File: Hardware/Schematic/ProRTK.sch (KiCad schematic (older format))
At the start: 37 parts

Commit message: Add files via upload
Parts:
- removed C? (x2): 1uF, symbol Device:C
- removed U?: AMS1117-3.3, Package_TO_SOT_SMD:SOT-223-3_TabPin2, symbol Regulator_Linear:AMS1117-3.3
- added 1PPS, RX_GNSS?, SCL_ALT, SCL_GNSS, SDA_ALT, SDA_GNSS, SYS_RSTN, TX_GNSS, WAKE-UP: TestPoint, symbol Connector:TestPoint
- added C? (x2): C, symbol Device:C
- added D?: SP0502BAJT, Package_TO_SOT_SMD:SOT-323_SC-70, symbol Power_Protection:SP0502BAJT
- added IC?: ST1S12GR, ASSETS:SOT95P280X110-5N, symbol Regular_Use:ST1S12GR
- added L?: L, symbol Device:L
- added R? (x3): R, symbol Device:R
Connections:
- net labels added: +3V3, 1PPS, RX_GNSS, SCL_ALT, SCL_GNSS, SCL_IMU, SDA_ALT, SDA_GNSS, SDA_IMU, SYS_RSTN, TX_GNSS, WAKE-UP
- net labels removed: SCL, SDA
- wire segments 92 -> 126
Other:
- moved on the sheet: 3.3V, CLK, CMD, CR2023, D+, D-, DAT0, DAT1, DAT2, DAT3, GND, VDD

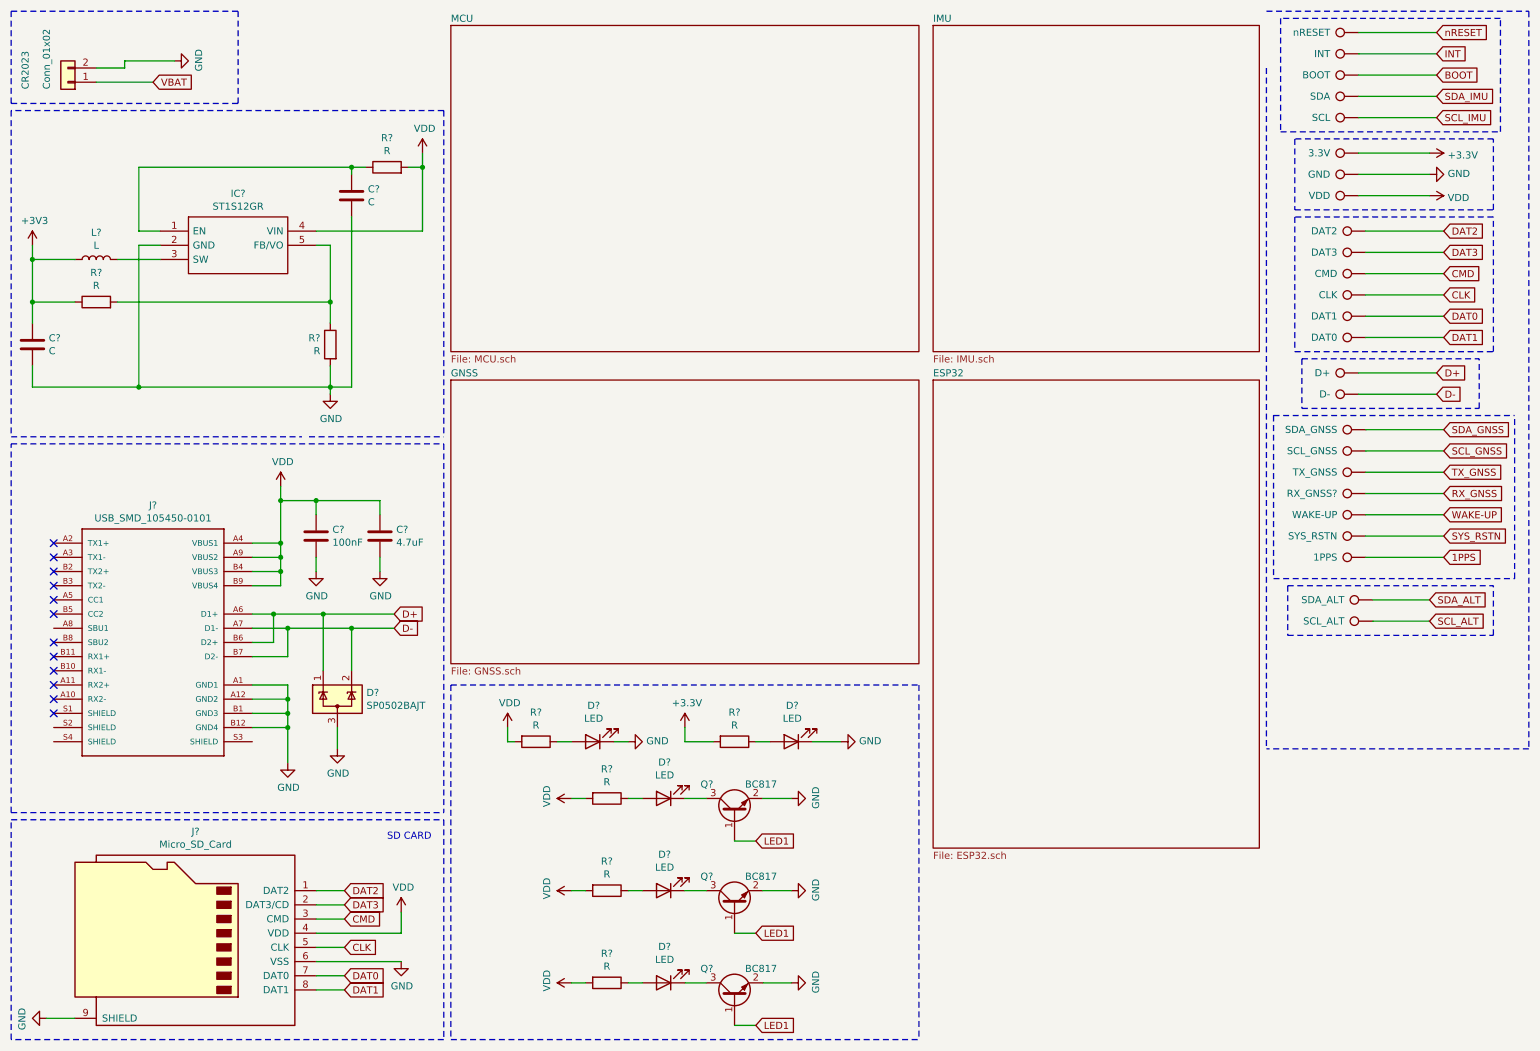
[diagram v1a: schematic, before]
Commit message: Add files via upload
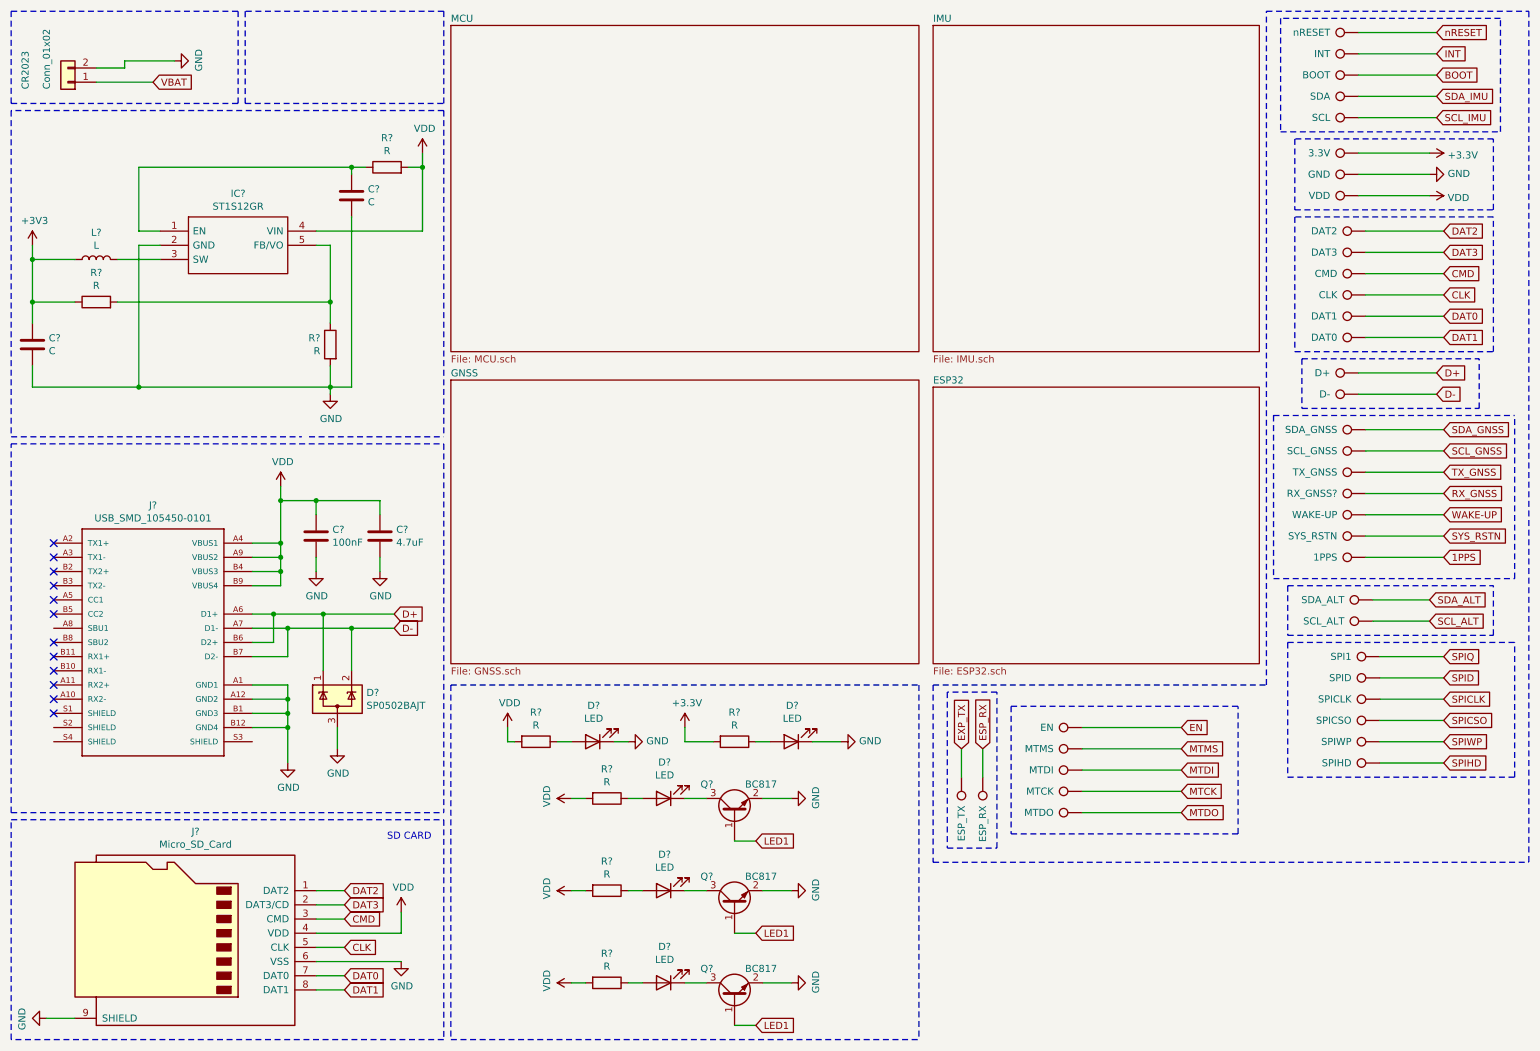
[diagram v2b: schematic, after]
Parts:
- added EN, ESP_RX, ESP_TX, MTCK, MTDI, MTDO, MTMS, SPI1, SPICLK, SPICSO, SPID, SPIHD, SPIWP: TestPoint, symbol Connector:TestPoint
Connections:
- new net EN: EN.1
- new net ESP_RX: ESP_RX.1
- new net EXP_TX: ESP_TX.1
- new net MTCK: MTCK.1
- new net MTDI: MTDI.1
- new net MTDO: MTDO.1
- new net MTMS: MTMS.1
- new net SPICLK: SPICLK.1
- new net SPICSO: SPICSO.1
- new net SPID: SPID.1
- new net SPIHD: SPIHD.1
- new net SPIQ: SPI1.1
- new net SPIWP: SPIWP.1
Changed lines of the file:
@@
 	9500 4550 10950 4550
 Wire Notes Line
-	11200 5700 9350 5700
-Wire Notes Line
-	9350 900  9350 5700
-Wire Notes Line
-	11200 500  11200 5700
+	11200 500  11200 6500
 $Sheet
-S 7000 3100 2300 3300
+S 7000 3150 2300 1950
 U 609C383C
 F0 "ESP32" 50
 F1 "ESP32.sch" 50
 $EndSheet
+Text GLabel 10600 5050 2    50   Input ~ 0
+SPIQ
+Text GLabel 10600 5200 2    50   Input ~ 0
+SPID
+Text GLabel 10600 5350 2    50   Input ~ 0
+SPICLK
+Text GLabel 10600 5500 2    50   Input ~ 0
+SPICSO
+Text GLabel 10600 5800 2    50   Input ~ 0
+SPIHD
+Text GLabel 10600 5650 2    50   Input ~ 0
+SPIWP
+Text GLabel 7200 5700 1    50   Input ~ 0
+EXP_TX
+Text GLabel 7350 5700 1    50   Input ~ 0
+ESP_RX
+Text GLabel 8750 5550 2    50   Input ~ 0
+EN
+Text GLabel 8750 5700 2    50   Input ~ 0
+MTMS
+Text GLabel 8750 5850 2    50   Input ~ 0
+MTDI
+Text GLabel 8750 6000 2    50   Input ~ 0
+MTCK
+Text GLabel 8750 6150 2    50   Input ~ 0
+MTDO
+$Comp
+L Connector:TestPoint SPID
+U 1 1 60B02F01
+P 10150 5200
+F 0 "SPID" V 10150 5400 50  0000 L CNN
+F 1 "TestPoint" V 10050 5150 50  0001 L CNN
+F 2 "" H 10350 5200 50  0001 C CNN
+F 3 "~" H 10350 5200 50  0001 C CNN
+	1    10150 5200
+	0    -1   -1   0
+$EndComp
+$Comp
+L Connector:TestPoint SPI1
+U 1 1 60B02F07
+P 10150 5050
+F 0 "SPI1" V 10150 5250 50  0000 L CNN
+F 1 "TestPoint" V 10050 5000 50  0001 L CNN
+F 2 "" H 10350 5050 50  0001 C CNN
+F 3 "~" H 10350 5050 50  0001 C CNN
+	1    10150 5050
+	0    -1   -1   0
+$EndComp
+$Comp
+L Connector:TestPoint SPICSO
+U 1 1 60B28901
+P 10150 5500
+F 0 "SPICSO" V 10150 5700 50  0000 L CNN
+F 1 "TestPoint" V 10050 5450 50  0001 L CNN
+F 2 "" H 10350 5500 50  0001 C CNN
+F 3 "~" H 10350 5500 50  0001 C CNN
+	1    10150 5500
+	0    -1   -1   0
+$EndComp
+$Comp
+L Connector:TestPoint SPICLK
+U 1 1 60B28907
+P 10150 5350
+F 0 "SPICLK" V 10150 5550 50  0000 L CNN
+F 1 "TestPoint" V 10050 5300 50  0001 L CNN
+F 2 "" H 10350 5350 50  0001 C CNN
+F 3 "~" H 10350 5350 50  0001 C CNN
+	1    10150 5350
+	0    -1   -1   0
+$EndComp
+$Comp
+L Connector:TestPoint SPIHD
+U 1 1 60B2E050
+P 10150 5800
+F 0 "SPIHD" V 10150 6000 50  0000 L CNN
+F 1 "TestPoint" V 10050 5750 50  0001 L CNN
+F 2 "" H 10350 5800 50  0001 C CNN
+F 3 "~" H 10350 5800 50  0001 C CNN
+	1    10150 5800
+	0    -1   -1   0
+$EndComp
+$Comp
+L Connector:TestPoint SPIWP
+U 1 1 60B2E056
+P 10150 5650
+F 0 "SPIWP" V 10150 5850 50  0000 L CNN
+F 1 "TestPoint" V 10050 5600 50  0001 L CNN
+F 2 "" H 10350 5650 50  0001 C CNN
+F 3 "~" H 10350 5650 50  0001 C CNN
+	1    10150 5650
+	0    -1   -1   0
+$EndComp
+Wire Wire Line
+	10150 5050 10600 5050
+Wire Wire Line
+	10600 5200 10150 5200
+Wire Wire Line
+	10150 5350 10600 5350
+Wire Wire Line
+	10600 5500 10150 5500
+Wire Wire Line
+	10150 5650 10600 5650
+Wire Wire Line
+	10150 5800 10600 5800
+Wire Notes Line
+	9500 5900 11100 5900
+Wire Notes Line
+	11100 5900 11100 4950
+Wire Notes Line
+	9500 4950 11100 4950
+Wire Notes Line
+	9500 4950 9500 5900
+Wire Notes Line
+	7000 5250 7000 6500
+Wire Notes Line
+	7000 6500 11200 6500
+Wire Notes Line
+	7000 5250 9350 5250
+Wire Notes Line
+	9350 5250 9350 500
+$Comp
+L Connector:TestPoint ESP_RX
+U 1 1 60B7FAB2
+P 7350 5900
+F 0 "ESP_RX" V 7350 6100 50  0000 L CNN
+F 1 "TestPoint" V 7250 5850 50  0001 L CNN
+F 2 "" H 7550 5900 50  0001 C CNN
+F 3 "~" H 7550 5900 50  0001 C CNN
+	1    7350 5900
+	-1   0    0    1
+$EndComp
+$Comp
+L Connector:TestPoint ESP_TX
+U 1 1 60B7FAB8
+P 7200 5900
+F 0 "ESP_TX" V 7200 6100 50  0000 L CNN
+F 1 "TestPoint" V 7100 5850 50  0001 L CNN
+F 2 "" H 7400 5900 50  0001 C CNN
+F 3 "~" H 7400 5900 50  0001 C CNN
+	1    7200 5900
+	-1   0    0    1
+$EndComp
+$Comp
+L Connector:TestPoint MTMS
+U 1 1 60B7FABE
+P 8050 5700
+F 0 "MTMS" V 8050 5900 50  0000 L CNN
+F 1 "TestPoint" V 7950 5650 50  0001 L CNN
+F 2 "" H 8250 5700 50  0001 C CNN
+F 3 "~" H 8250 5700 50  0001 C CNN
+	1    8050 5700
+	0    -1   -1   0
+$EndComp
+$Comp
+L Connector:TestPoint EN
+U 1 1 60B7FAC4
+P 8050 5550
+F 0 "EN" V 8050 5750 50  0000 L CNN
+F 1 "TestPoint" V 7950 5500 50  0001 L CNN
+F 2 "" H 8250 5550 50  0001 C CNN
+F 3 "~" H 8250 5550 50  0001 C CNN
+	1    8050 5550
+	0    -1   -1   0
+$EndComp
+$Comp
+L Connector:TestPoint MTCK
+U 1 1 60B7FACA
+P 8050 6000
+F 0 "MTCK" V 8050 6200 50  0000 L CNN
+F 1 "TestPoint" V 7950 5950 50  0001 L CNN
+F 2 "" H 8250 6000 50  0001 C CNN
+F 3 "~" H 8250 6000 50  0001 C CNN
+	1    8050 6000
+	0    -1   -1   0
+$EndComp
+$Comp
+L Connector:TestPoint MTDI
+U 1 1 60B7FAD0
+P 8050 5850
+F 0 "MTDI" V 8050 6050 50  0000 L CNN
+F 1 "TestPoint" V 7950 5800 50  0001 L CNN
+F 2 "" H 8250 5850 50  0001 C CNN
+F 3 "~" H 8250 5850 50  0001 C CNN
+	1    8050 5850
+	0    -1   -1   0
+$EndComp
+Wire Wire Line
+	7200 5900 7200 5700
+Wire Wire Line
+	7350 5700 7350 5900
+Wire Notes Line
+	7450 5300 7100 5300
+Wire Notes Line
+	7100 5300 7100 6400
+Wire Notes Line
+	7100 6400 7450 6400
+Wire Notes Line
+	7450 6400 7450 5300
+$Comp
+L Connector:TestPoint MTDO
+U 1 1 60BAB95C
+P 8050 6150
+F 0 "MTDO" V 8050 6350 50  0000 L CNN
+F 1 "TestPoint" V 7950 6100 50  0001 L CNN
+F 2 "" H 8250 6150 50  0001 C CNN
+F 3 "~" H 8250 6150 50  0001 C CNN
+	1    8050 6150
+	0    -1   -1   0
+$EndComp
+Wire Wire Line
+	8750 5550 8050 5550
+Wire Wire Line
+	8050 5700 8750 5700
+Wire Wire Line
+	8050 5850 8750 5850
+Wire Wire Line
+	8050 6000 8750 6000
+Wire Wire Line
+	8050 6150 8750 6150
+Wire Notes Line
+	9150 6300 9150 5400
+Wire Notes Line
+	7550 5400 7550 6300
+Wire Notes Line
+	7550 6300 9150 6300
+Wire Notes Line
+	7550 5400 9150 5400
+Wire Notes Line
+	2150 500  2150 1150
+Wire Notes Line
+	2150 1150 3550 1150
+Wire Notes Line
+	3550 1150 3550 500
+Wire Notes Line
+	3550 500  2150 500
 $EndSCHEMATC
